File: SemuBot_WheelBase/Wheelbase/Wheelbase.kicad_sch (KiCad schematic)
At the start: 39 parts, among them IC1 NCP164CSN330T1G, J1 10155435-00011LF, J10 B5B-XH-A_LF__SN_, J11 B5B-XH-A_LF__SN_, J12 B5B-XH-A_LF__SN_, J13 SSW-104-01-FM-D, J3 TB003-500-P02BE, J4 B5B-XH-A_LF__SN_, J5 B5B-XH-A_LF__SN_, J6 B5B-XH-A_LF__SN_, J7 1984620, J8 1984620, J9 1984620, U1 STM32F303RET6, Y2 X322516MLB4SI

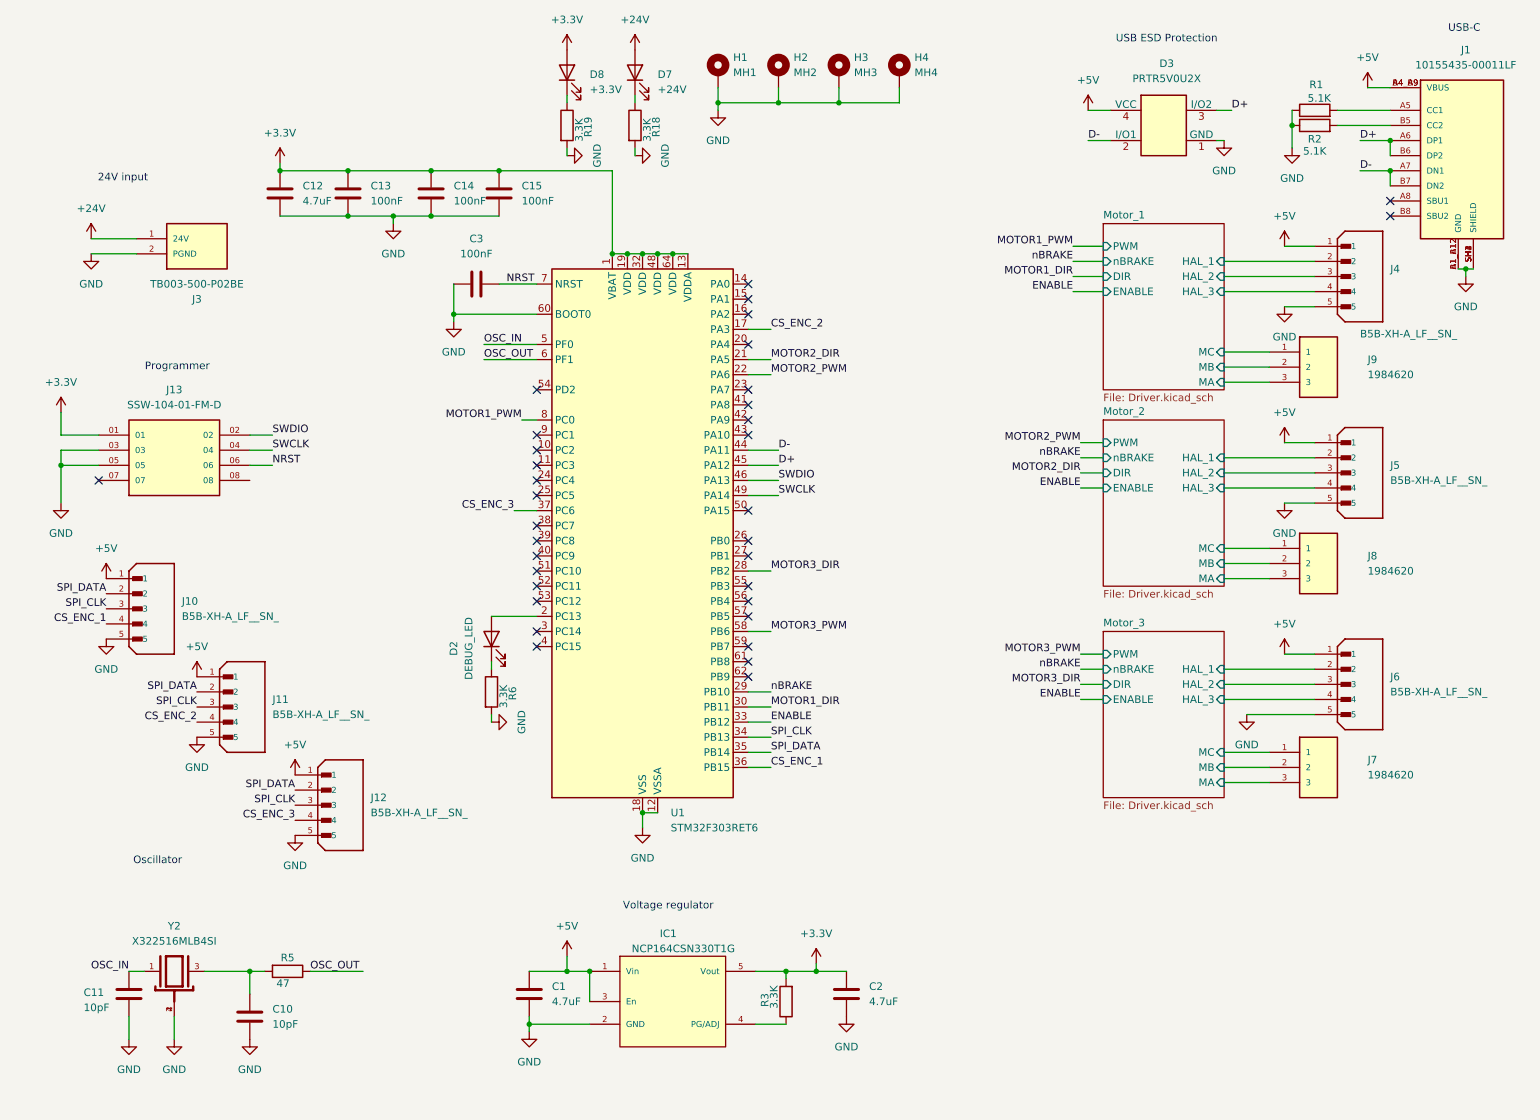
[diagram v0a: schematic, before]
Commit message: Updating board
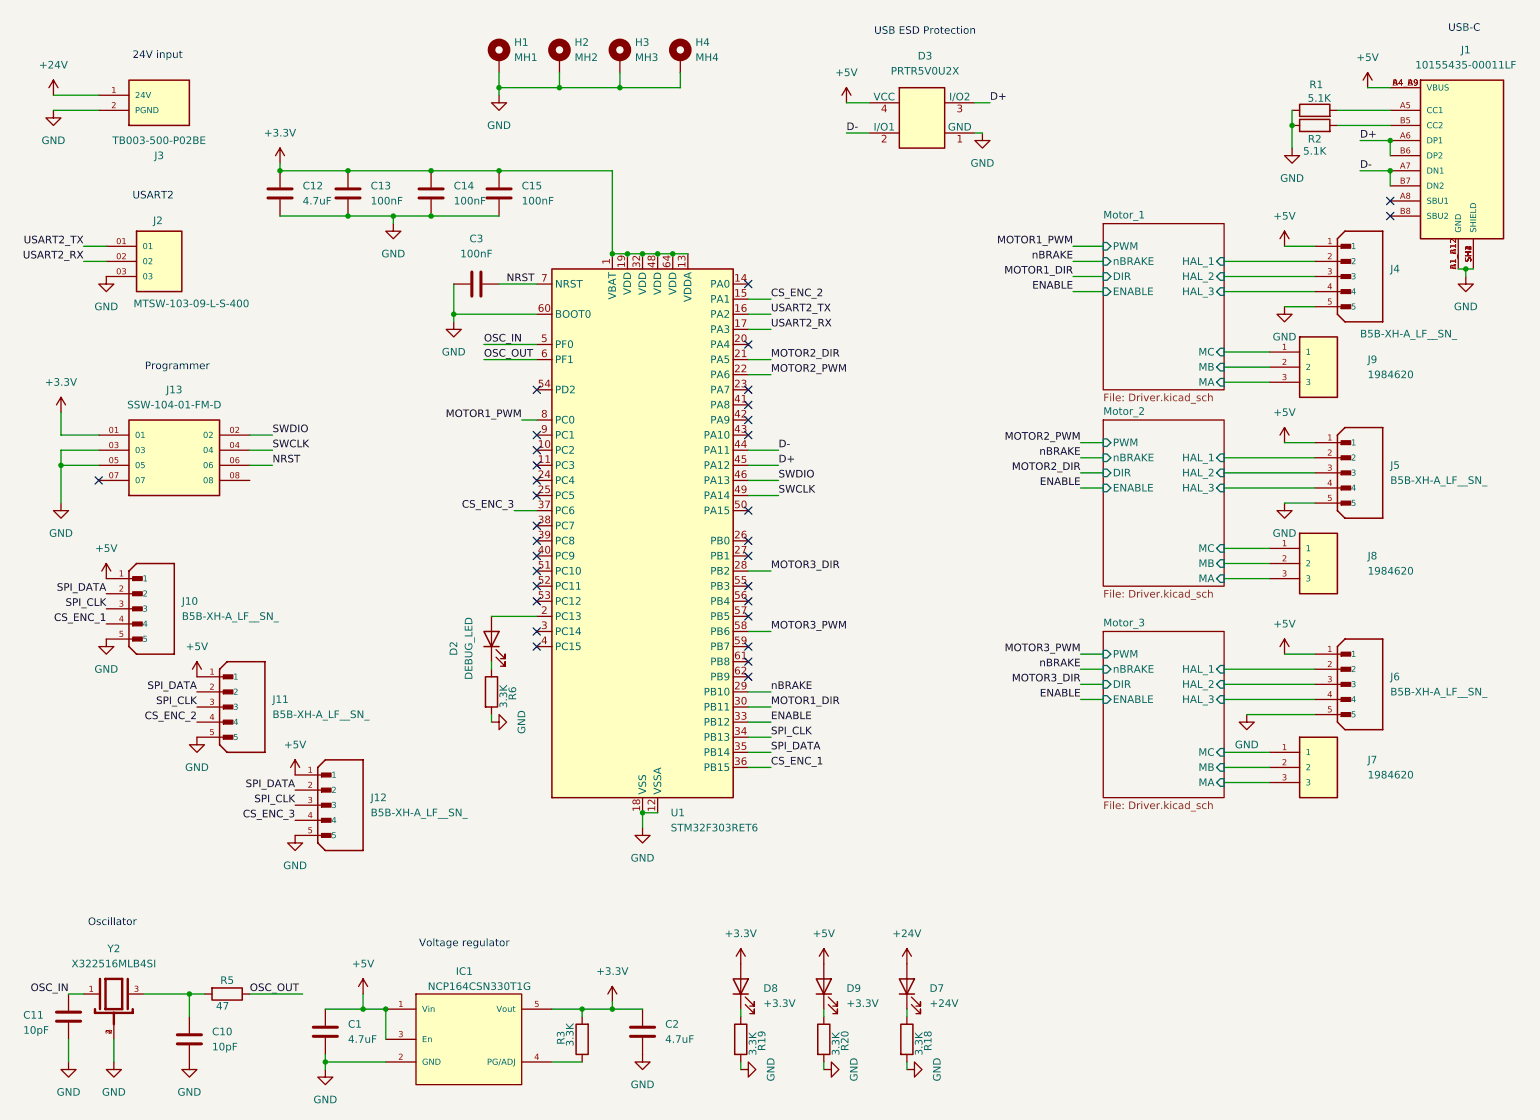
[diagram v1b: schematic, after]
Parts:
- added D9: +3.3V, LED_SMD:LED_0603_1608Metric_Pad1.05x0.95mm_HandSolder, symbol Device:LED
- added J2: MTSW-103-09-L-S-400, MTSW-103-09-L-S-400:SAMTEC_MTSW-103-09-L-S-400, symbol MTSW-103-09-L-S-400:MTSW-103-09-L-S-400
- added R20: 3.3K, Resistor_SMD:R_0603_1608Metric_Pad0.98x0.95mm_HandSolder, symbol Device:R
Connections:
- net +5V: now also D9.2 (A)
- net CS_ENC_2: now also U1.15 (PA1); no longer U1.17 (PA3)
- net GND: now also J2.03, R20.2
- net USART2_TX: now reaches U1.16 (PA2)
- net USART2_TX: now also J2.01
- new net: D9.1 (K), R20.1
- new net USART2_RX: J2.02, U1.17 (PA3)
- no-connect marks 34 -> 32
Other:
- note added: "USART2"
- moved on the sheet: C1, C10, C11, C2, D3, D7, D8, H1, H2, H3, H4, IC1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
